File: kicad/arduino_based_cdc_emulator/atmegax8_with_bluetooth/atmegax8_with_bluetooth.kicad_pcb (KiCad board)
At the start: 2 copper layers, 40.9 x 35.7 mm, 70 parts, among them IC1 ATMEGA88-A, P1 CONN_9, P2 SPI, P3 CONN_4, Q1 BC817-40, U1 78L05, U2 F-6188, U3 LM358, Y1 Crystal_GND2

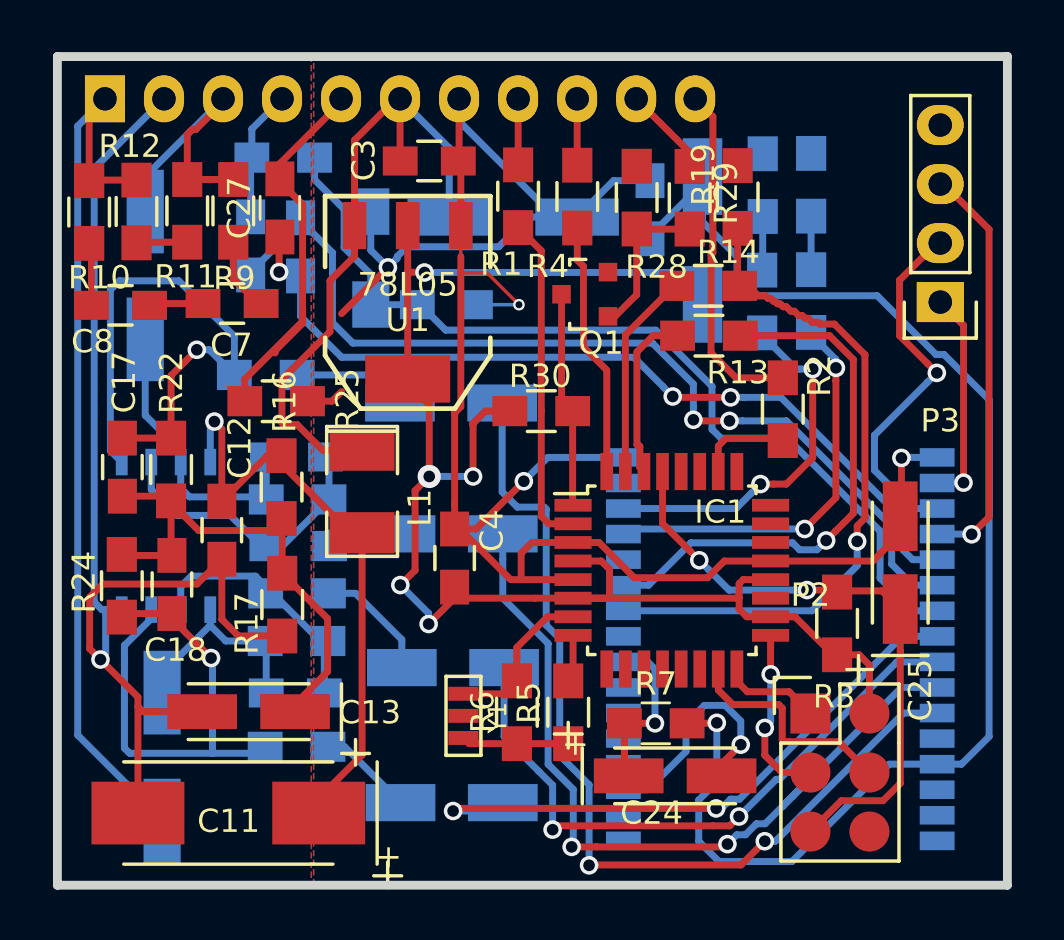
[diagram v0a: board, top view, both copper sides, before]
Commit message: update
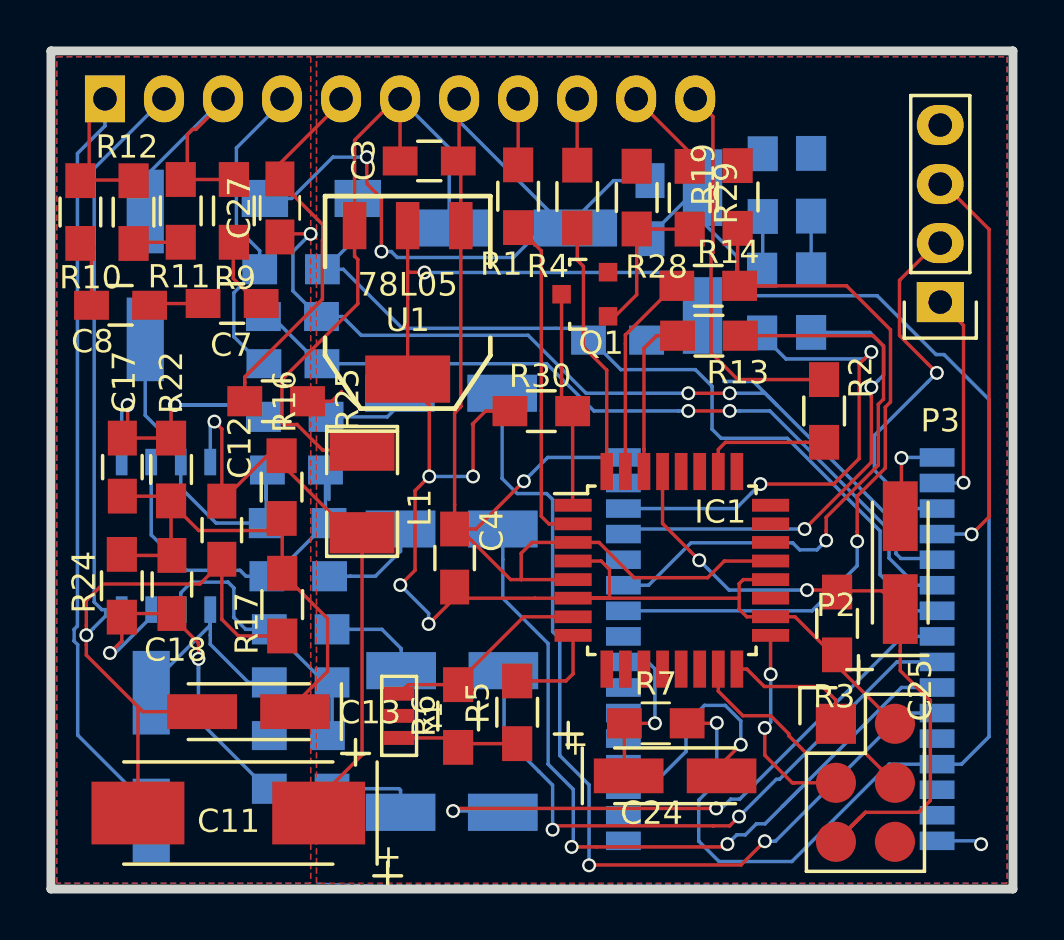
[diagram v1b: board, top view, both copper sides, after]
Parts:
- moved C28 7.52 mm to (93.7, 149.1)
- moved C23 5.39 mm to (79.8, 150.1), turned to 180 degrees
- moved R27 4.82 mm to (79.7, 146.1)
- moved C22 3.62 mm to (80.5, 143.0), turned to 180 degrees
- moved C26 3.02 mm to (79.7, 148.1), turned to 0 degrees
- moved Y1 2.77 mm to (84.3, 166.2)
- moved R6 2.53 mm to (86.9, 165.3)
- moved R5 2.20 mm to (89.4, 165.1)
- moved R20 2.19 mm to (79.8, 152.4)
- moved C16 1.84 mm to (80.0, 166.1)
- moved R23 1.81 mm to (80.1, 168.4)
- moved R18 1.79 mm to (80.1, 163.8)
- moved R2 1.78 mm to (102.6, 152.1)
- moved R8 1.56 mm to (80.1, 161.5)
- moved R21 1.30 mm to (80.0, 159.3)
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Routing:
- net Net-(C17-Pad1): track 24.2 -> 15.4 mm, vias 1 -> 2
- net /MIC_IN2: track 6.42 -> 14.5 mm
- net /MICP: track 41.6 -> 34.5 mm
- net GND: track 103.9 -> 97.8 mm, vias 5 -> 6
- net /LED2: track 15.7 -> 21.2 mm
- net Net-(C18-Pad1): track 21.7 -> 17.1 mm, vias 1 -> 2
- net Net-(C15-Pad2): track 12.6 -> 16.7 mm
- net /ARESET: track 26.7 -> 30.7 mm
- net Net-(C15-Pad1): track 13.6 -> 17.1 mm
- net /MICN: track 36.8 -> 40.1 mm
- net /LED1: track 17.3 -> 20.5 mm
- net TX: track 29.2 -> 31.4 mm
- net RX: track 23.3 -> 25.5 mm
- net Net-(IC1-Pad8): track 2.04 -> 4.18 mm
- net Net-(C14-Pad1): track 9.36 -> 11.4 mm
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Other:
- board size 40.9 x 35.7 mm -> 41.4 x 36.1 mm
- net class Default: clearance 0.2 -> 0.15; via_dia 0.5 -> 0.6; via_drill 0.3 -> 0.4
- rule trace_clearance: 0.2 -> 0.15
